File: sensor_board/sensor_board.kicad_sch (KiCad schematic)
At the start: 20 parts, among them J1 Conn_02x20_Odd_Even, U1 BME280, U2 MPU-6050

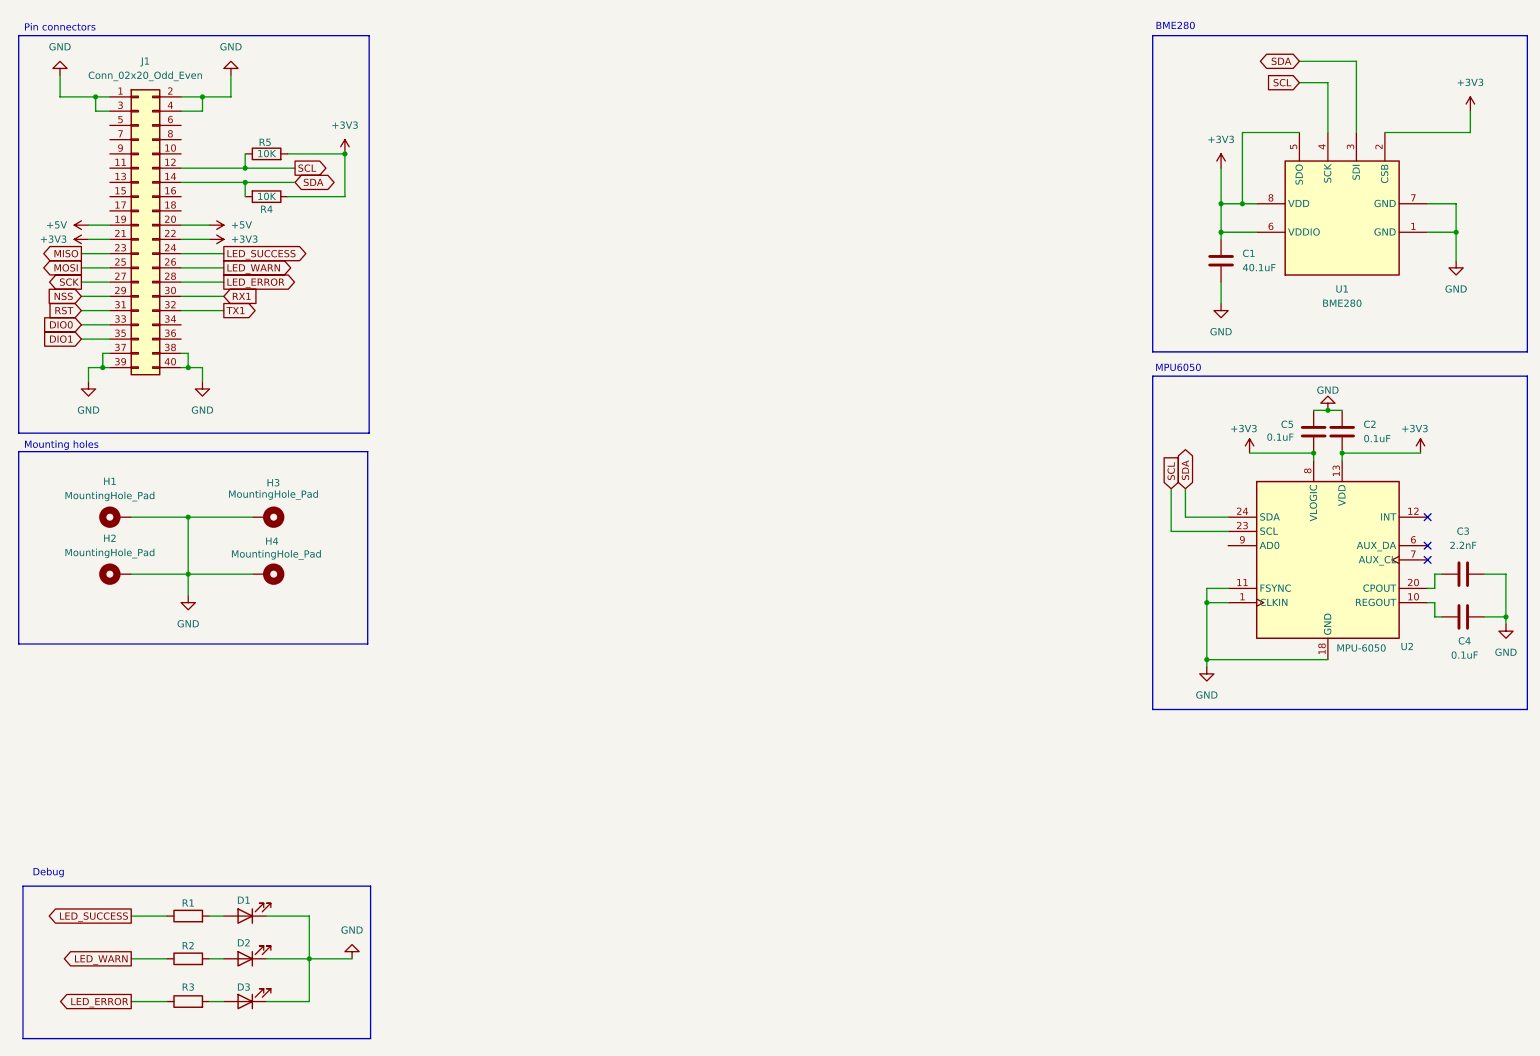
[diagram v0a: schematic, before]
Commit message: sensor board
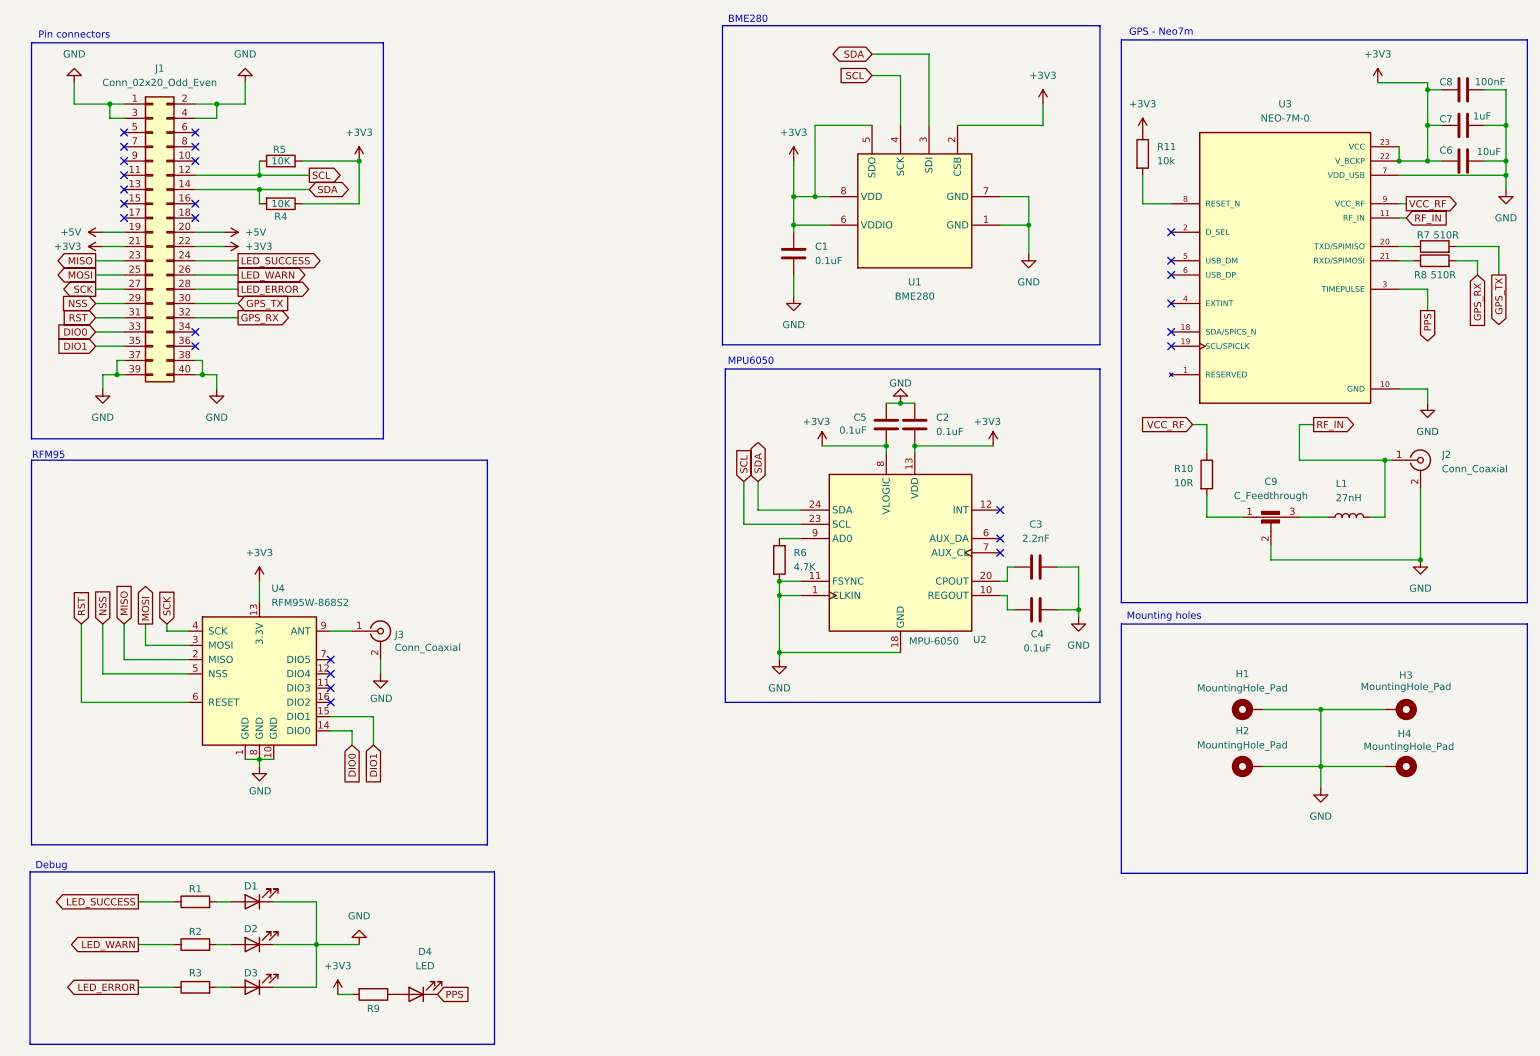
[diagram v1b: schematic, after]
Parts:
- added C6: 10uF, symbol Device:C
- added C7: 1uF, symbol Device:C
- added C8: 100nF, symbol Device:C
- added C9: C_Feedthrough, symbol Device:C_Feedthrough
- added D4: LED, symbol Device:LED
- added J2: Conn_Coaxial, Connector_Coaxial:U.FL_Hirose_U.FL-R-SMT-1_Vertical, symbol Connector:Conn_Coaxial
- added J3: Conn_Coaxial, Connector_Coaxial:SMA_Amphenol_132134-11_Vertical, symbol Connector:Conn_Coaxial
- added L1: 27nH, symbol Device:L
- added R10: 10R, symbol Device:R
- added R11: 10k, symbol Device:R
- added R6: 4.7K, symbol Device:R
- added R7, R8: 510R, symbol Device:R
- added R9: R, symbol Device:R
- added U3: NEO-7M-0, NEO-7M-0:XCVR_NEO-7M-0, symbol NEO-7M-0:NEO-7M-0
- added U4: RFM95W-868S2, symbol RF_Module:RFM95W-868S2
- C1: value 40.1uF -> 0.1uF
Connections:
- net +3V3: now also C6.1, C7.1, C8.1, R11.1, R9.2, U3.22 (V_BCKP), U3.23 (VCC), U4.13 (3.3V)
- net DIO0: now also U4.14 (DIO0)
- net DIO1: now also U4.15 (DIO1)
- net GND: now also C6.2, C7.2, C8.2, C9.2, J2.2 (Ext), J3.2 (Ext), R6.1, U3.10 (GND), U3.12 (GND), U3.13 (GND), U3.24 (GND), U3.7 (VDD_USB), U4.1 (GND), U4.10 (GND), U4.8 (GND)
- net MISO: now also U4.2 (MISO)
- net MOSI: now also U4.3 (MOSI)
- net NSS: now also U4.5 (NSS)
- net RST: now also U4.6 (RESET)
- net SCK: now also U4.4 (SCK)
- net at U2.9 (AD0): now also R6.2
- net RX1 renamed GPS_TX
- net GPS_TX: now also R7.2
- net TX1 renamed GPS_RX
- net GPS_RX: now also R8.2
- new net: J3.1 (In), U4.9 (ANT)
- new net: R11.2, U3.8 (RESET_N)
- new net: C9.1, R10.2
- new net: C9.3, L1.1
- new net: U3.1 (RESERVED), U3.14 (RESERVED), U3.15 (RESERVED), U3.16 (RESERVED), U3.17 (RESERVED)
- new net: R7.1, U3.20 (TXD/SPIMISO)
- new net: R8.1, U3.21 (RXD/SPIMOSI)
- new net: D4.2 (A), R9.1
- new net PPS: D4.1 (K), U3.3 (TIMEPULSE)
- new net RF_IN: J2.1 (In), L1.2, U3.11 (RF_IN)
- new net VCC_RF: R10.1, U3.9 (VCC_RF)
- no-connect marks 3 -> 27
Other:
- note added: "GPS - Neo7m"
- note added: "RFM95"
- moved on the sheet: C1, C2, C3, C4, C5, D1, D2, D3, H1, H2, H3, H4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

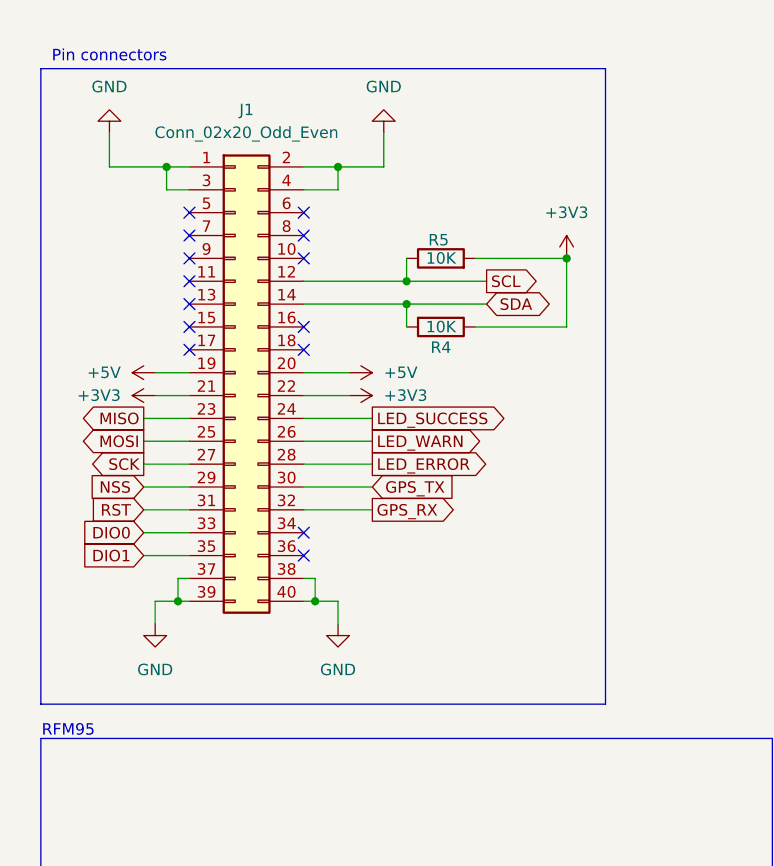
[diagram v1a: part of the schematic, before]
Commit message: sensor
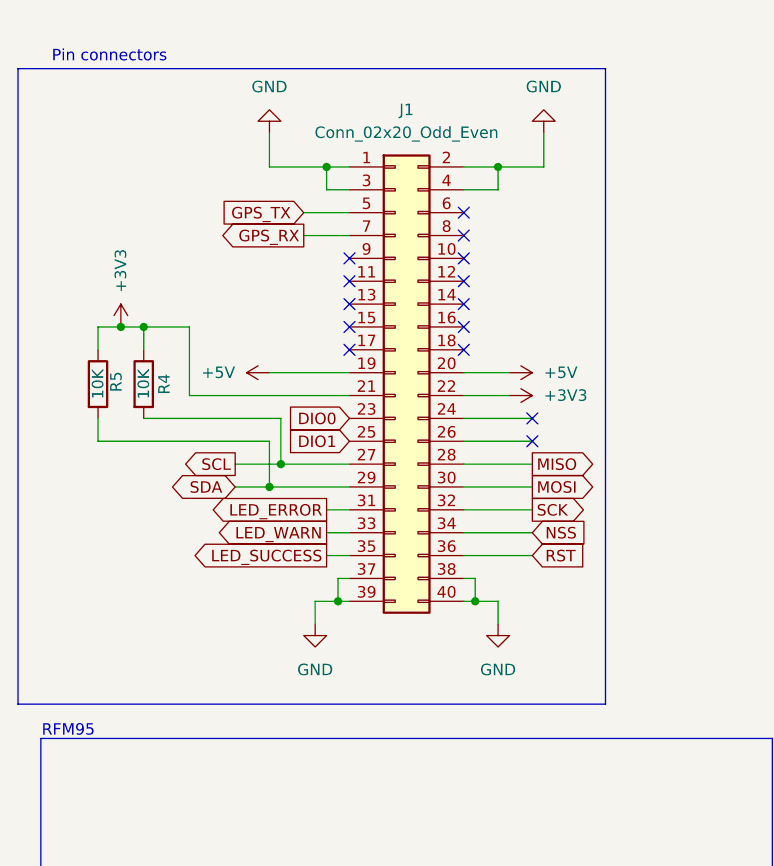
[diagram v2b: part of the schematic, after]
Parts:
- C1, C2, C3, C4, C5, C6, C7, C8: footprint (none) -> Capacitor_SMD:C_0805_2012Metric
- C9: footprint (none) -> Filter:Filter_Mini-Circuits_FV1206-7
- D1, D2, D3, D4: footprint (none) -> LED_THT:LED_D8.0mm
- H1, H2, H3, H4: footprint (none) -> MountingHole:MountingHole_3.2mm_M3_DIN965_Pad
- J1: footprint (none) -> Connector_PinSocket_2.54mm:PinSocket_2x20_P2.54mm_Vertical
- L1: footprint (none) -> Inductor_SMD:L_0603_1608Metric
- R1, R2, R3: value R -> 220; footprint (none) -> Resistor_SMD:R_0603_1608Metric
- R10, R11, R4, R5, R6, R7, R8: footprint (none) -> Resistor_SMD:R_0603_1608Metric
- R9: value R -> 220R; footprint (none) -> Resistor_SMD:R_0603_1608Metric
- U4: footprint (none) -> RF_Module:HOPERF_RFM9XW_SMD
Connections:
- net +3V3: now also R5.1; no longer R5.2
- net DIO0: now also J1.23 (Pin_23); no longer J1.33 (Pin_33)
- net DIO1: now also J1.25 (Pin_25); no longer J1.35 (Pin_35)
- net GPS_RX: now also J1.7 (Pin_7); no longer J1.32 (Pin_32)
- net GPS_TX: now also J1.5 (Pin_5); no longer J1.30 (Pin_30)
- net LED_ERROR: now also J1.31 (Pin_31); no longer J1.28 (Pin_28)
- net LED_SUCCESS: now also J1.35 (Pin_35); no longer J1.24 (Pin_24)
- net LED_WARN: now also J1.33 (Pin_33); no longer J1.26 (Pin_26)
- net MISO: now also J1.28 (Pin_28); no longer J1.23 (Pin_23)
- net MOSI: now also J1.30 (Pin_30); no longer J1.25 (Pin_25)
- net NSS: now also J1.34 (Pin_34); no longer J1.29 (Pin_29)
- net RST: now also J1.36 (Pin_36); no longer J1.31 (Pin_31)
- net SCK: now also J1.32 (Pin_32); no longer J1.27 (Pin_27)
- net SCL: now also J1.27 (Pin_27), R4.2; no longer J1.12 (Pin_12), R5.1
- net SDA: now also J1.29 (Pin_29), R5.2; no longer J1.14 (Pin_14), R4.2
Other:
- moved on the sheet: J1, R4, R5
